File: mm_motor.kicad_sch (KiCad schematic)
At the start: 2 parts, among them J2 Conn_01x06_Pin, M1 N20_encoder

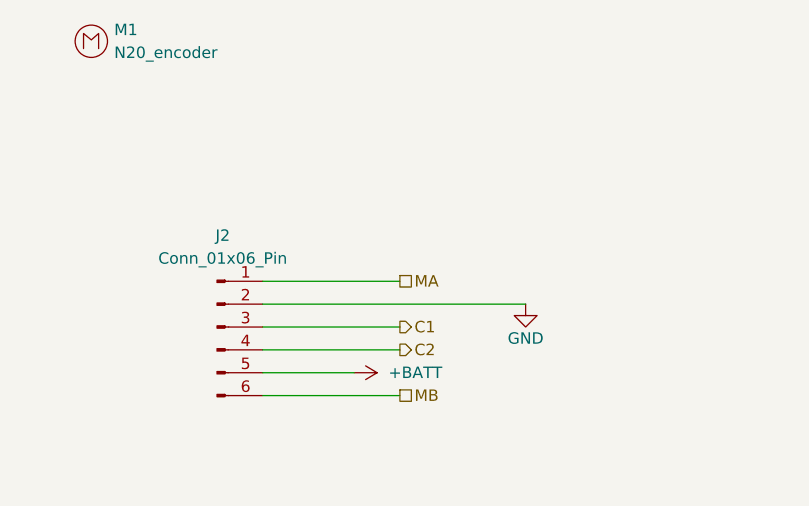
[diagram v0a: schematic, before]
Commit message: nadjibmarouen
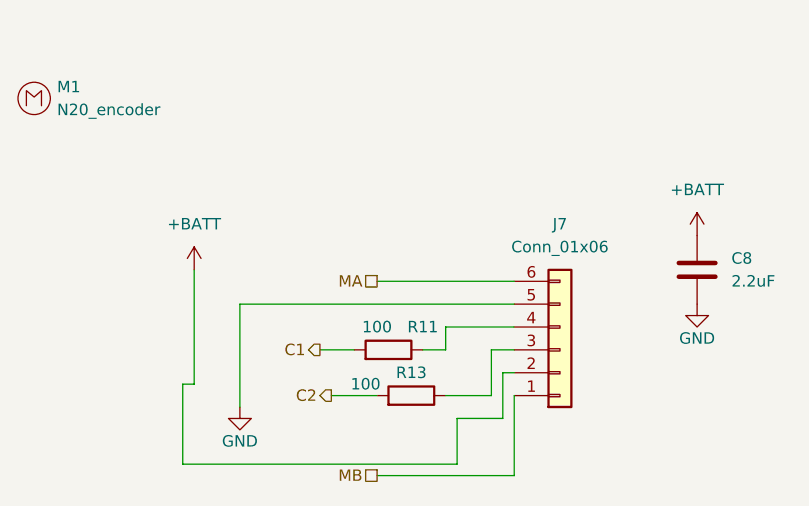
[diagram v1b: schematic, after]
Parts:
- removed J2: Conn_01x06_Pin, symbol Connector:Conn_01x06_Pin
- added C8: 2.2uF, Capacitor_SMD:C_0603_1608Metric, symbol Device:C
- added J7: Conn_01x06, Connector_PinHeader_2.54mm:PinHeader_1x06_P2.54mm_Vertical, symbol Connector_Generic:Conn_01x06
- added R11, R13: 100, Resistor_SMD:R_0603_1608Metric, symbol Device:R
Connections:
- net +BATT: now also C8.1, J7.2 (Pin_2)
- net C1: now also R11.2
- net C2: now also R13.2
- net GND: now also C8.2, J7.5 (Pin_5)
- net MA: now also J7.6 (Pin_6)
- net MB: now also J7.1 (Pin_1)
- new net: J7.4 (Pin_4), R11.1
- new net: J7.3 (Pin_3), R13.1
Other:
- moved on the sheet: M1
